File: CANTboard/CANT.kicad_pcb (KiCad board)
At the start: 2 copper layers, 67.6 x 50.8 mm, 63 parts, among them J1 Conn_02x08_Odd_Even, J2 Screw_Terminal_01x02, J3 Screw_Terminal_01x04, J4 USB_C_Receptacle_USB2.0, P2 SWD, SW1 SW_SPST, U1 USBLC6-2SC6, U2 SN74LVC1G14DBV, U3 ST485EBDR, U4 LD1117S33TR, U5 STM32H743VITx, U6 MCP2558FD-xSN, U7 74LVC1G66, U8 MCP2558FD-xSN, U9 74LVC1G66, Y1 Crystal

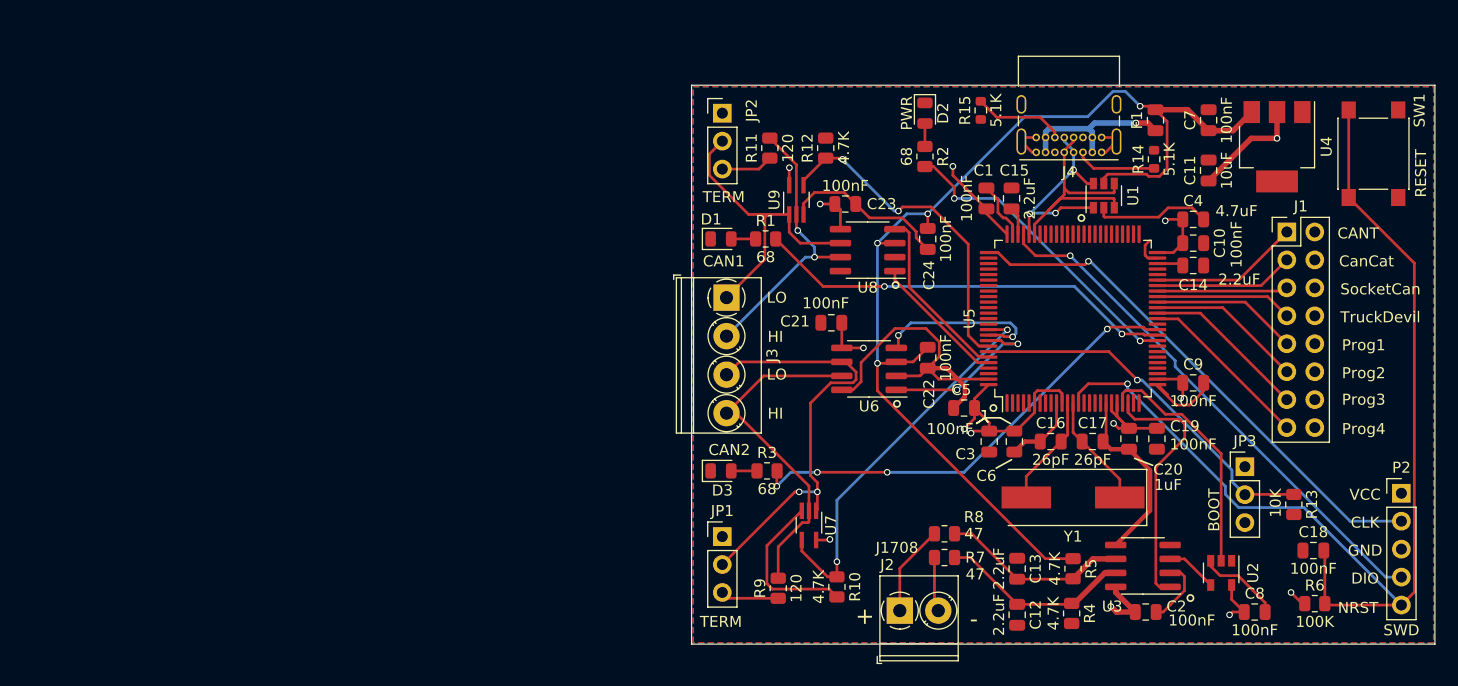
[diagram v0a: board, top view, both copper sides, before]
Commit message: Everything routed, commiting before last check before ordering PCBs
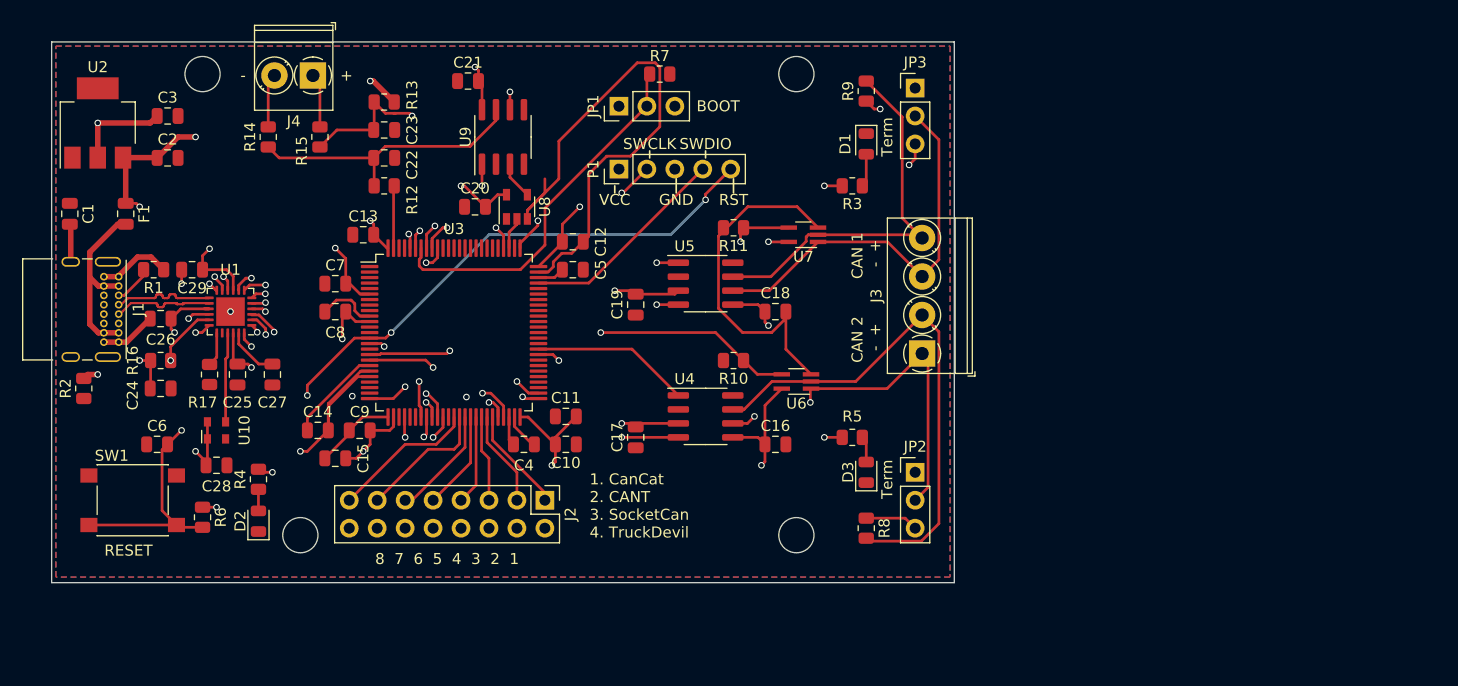
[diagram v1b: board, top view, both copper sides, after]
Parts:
- removed P2: SWD, Connector_PinHeader_2.54mm:PinHeader_1x05_P2.54mm_Vertical
- removed Y1: Crystal, Crystal:Crystal_SMD_HC49-SD
- added  : MountingHole_3.2mm_M3, MountingHole:MountingHole_3.2mm_M3, F.Cu at (37.5, 107.3)
- added  : MountingHole_3.2mm_M3, MountingHole:MountingHole_3.2mm_M3, F.Cu at (82.5, 107.3)
- added  : MountingHole_3.2mm_M3, MountingHole:MountingHole_3.2mm_M3, F.Cu at (82.5, 65.4)
- added  : MountingHole_3.2mm_M3, MountingHole:MountingHole_3.2mm_M3, F.Cu at (28.6, 65.4)
- added C25: 100nF, Capacitor_SMD:C_0805_2012Metric, F.Cu at (31.8, 92.7)
- added C26: 1uF, Capacitor_SMD:C_0805_2012Metric, F.Cu at (24.8, 87.6)
- added C27: 1uF, Capacitor_SMD:C_0805_2012Metric, F.Cu at (34.9, 92.7)
- added C28: 100nF, Capacitor_SMD:C_0805_2012Metric, F.Cu at (29.8, 101.0)
- added C29: 100nF, Capacitor_SMD:C_0805_2012Metric, F.Cu at (27.6, 83.2)
- added P1: SWD, Connector_PinHeader_2.54mm:PinHeader_1x05_P2.54mm_Vertical, F.Cu at (66.4, 74.0)
- added R16: 20K, Resistor_SMD:R_0805_2012Metric, F.Cu at (24.8, 91.4)
- added R17: 8.06K, Resistor_SMD:R_0805_2012Metric, F.Cu at (29.2, 92.7)
- added U10: DSC1001, DSC1001:Oscillator_SMD_Microchip_DSC1001-4Pin_2.5x2.0mm, F.Cu at (29.8, 97.8)
- C1: value 100nF -> 1uF
- C11: value 10uF -> 4.7uF
- C12, C13, C14: value 2.2uF -> 100nF
- C15: value 2.2uF -> 1uF
- C16, C17: value 26pF -> 100nF
- C20: value 1uF -> 100nF
- C22, C23, C5: value 100nF -> 2.2uF
- C24: value 100nF -> 4.7uF
- C3: value 100nF -> 10uF
- C4: value 4.7uF -> 2.2uF
- J1: value Conn_02x08_Odd_Even -> USB_C_Receptacle_USB2.0; footprint Connector_PinHeader_2.54mm:PinHeader_2x08_P2.54mm_Vertical -> Connector_USB:USB_C_Receptacle_GCT_USB4085
- J2: value Screw_Terminal_01x02 -> Conn_02x08_Odd_Even; footprint TerminalBlock_Phoenix:TerminalBlock_Phoenix_PT-1,5-2-3.5-H_1x02_P3.50mm_Horizontal -> Connector_PinHeader_2.54mm:PinHeader_2x08_P2.54mm_Vertical
- J4: value USB_C_Receptacle_USB2.0 -> Screw_Terminal_01x02; footprint Connector_USB:USB_C_Receptacle_GCT_USB4085 -> TerminalBlock_Phoenix:TerminalBlock_Phoenix_PT-1,5-2-3.5-H_1x02_P3.50mm_Horizontal
- R1, R2: value 68 -> 5.1K
- R11: value 120 -> 4.7K
- R13: value 10k -> 4.7K
- R14, R15: value 5.1K -> 47; footprint Resistor_SMD:R_0603_1608Metric -> Resistor_SMD:R_0805_2012Metric
- R4, R5: value 4.7K -> 68
- R7: value 47 -> 10k
- R8: value 47 -> 120
- U1: value USBLC6-2SC6 -> USB3343; footprint Package_TO_SOT_SMD:SOT-23-6 -> Package_DFN_QFN:QFN-24-1EP_4x4mm_P0.5mm_EP2.6x2.6mm
- U2: value SN74LVC1G14DBV -> LD1117S33TR; footprint Package_TO_SOT_SMD:SOT-23-5 -> Package_TO_SOT_SMD:SOT-223
- U3: value ST485EBDR -> STM32H743VITx; footprint Package_SO:SOIC-8_3.9x4.9mm_P1.27mm -> Package_QFP:LQFP-100_14x14mm_P0.5mm
- U4: value LD1117S33TR -> MCP2558FD-xSN; footprint Package_TO_SOT_SMD:SOT-223 -> Package_SO:SOIC-8_3.9x4.9mm_P1.27mm
- U5: value STM32H743VITx -> MCP2558FD-xSN; footprint Package_QFP:LQFP-100_14x14mm_P0.5mm -> Package_SO:SOIC-8_3.9x4.9mm_P1.27mm
- U6: value MCP2558FD-xSN -> 74LVC1G66; footprint Package_SO:SOIC-8_3.9x4.9mm_P1.27mm -> Package_TO_SOT_SMD:SOT-353_SC-70-5_Handsoldering
- U8: value MCP2558FD-xSN -> SN74LVC1G14DBV; footprint Package_SO:SOIC-8_3.9x4.9mm_P1.27mm -> Package_TO_SOT_SMD:SOT-23-5
- U9: value 74LVC1G66 -> ST485EBDR; footprint Package_TO_SOT_SMD:SOT-353_SC-70-5_Handsoldering -> Package_SO:SOIC-8_3.9x4.9mm_P1.27mm
- moved SW1 117.1 mm to (22.2, 104.1), turned to 0 degrees
- moved U2 110.0 mm to (19.1, 69.8), turned to 90 degrees
- moved J1 106.2 mm to (21.0, 83.8), turned to 270 degrees
- moved R6 101.4 mm to (28.6, 105.7), turned to 270 degrees
- moved C2 98.0 mm to (25.4, 73.0), turned to 0 degrees
- moved F1 94.0 mm to (21.6, 78.1), turned to 270 degrees
- moved R13 90.4 mm to (45.1, 67.9), turned to 180 degrees
- moved C8 87.9 mm to (40.6, 87.0)
- moved C1 83.3 mm to (16.5, 78.1), turned to 270 degrees
- moved G*** 82.4 mm to (33.0, 85.7)
- moved C14 81.0 mm to (39.1, 97.8)
- moved C7 80.8 mm to (40.6, 84.5), turned to 0 degrees
- moved R14 80.5 mm to (34.5, 71.1)
- moved C3 80.3 mm to (25.4, 69.2), turned to 0 degrees
- moved U1 80.1 mm to (31.1, 87.0), turned to 180 degrees
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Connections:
- C1 pad 1: VCC -> GND
- C1 pad 2: GND -> Net-(C1-Pad2)
- C10 pad 1: VCC -> GND
- C10 pad 2: GND -> VCC
- C11 pad 1: VCC -> GND
- C11 pad 2: GND -> VCC
- C12 pad 1: Net-(C12-Pad1) -> GND
- C12 pad 2: GND -> VCC
- C13 pad 2: Net-(C13-Pad2) -> VCC
- C14 pad 1: Net-(C14-Pad1) -> GND
- C14 pad 2: GND -> VCC
- C15 pad 1: Net-(C15-Pad1) -> GND
- C15 pad 2: GND -> VCC
- C16 pad 1: GND -> VCC
- C16 pad 2: Net-(C16-Pad2) -> GND
- C17 pad 1: Net-(C17-Pad1) -> GND
- C17 pad 2: GND -> VBUS
- C18 pad 1: GND -> VCC
- C18 pad 2: /NRST -> GND
- C19 pad 2: VCC -> VBUS
- C2 pad 1: GND -> VBUS
- C2 pad 2: VCC -> GND
- C22 pad 1: GND -> Net-(C22-Pad1)
- C22 pad 2: VBUS -> GND
- C23 pad 2: VCC -> Net-(C23-Pad2)
- C4 pad 1: VCC -> Net-(C4-Pad1)
- C5 pad 1: VCC -> Net-(C5-Pad1)
- C6 pad 1: VCC -> GND
- C6 pad 2: GND -> /Microcontroller/NRST
- C7 pad 1: VBUS -> GND
- C7 pad 2: GND -> VCC
- C8 pad 1: VCC -> GND
- C8 pad 2: GND -> VCC
- C9 pad 1: VCC -> GND
- C9 pad 2: GND -> VCC
- F1 pad 1: Net-(F1-Pad1) -> VBUS
- F1 pad 2: VBUS -> Net-(F1-Pad2)
- J2 pad 2: Net-(J2-Pad2) -> VCC
- J3 pad 1: CAN1_L -> CAN3_L
- J3 pad 2: CAN1_H -> CAN3_H
- J3 pad 3: CAN2_L -> CAN1_L
- J3 pad 4: CAN2_H -> CAN1_H
- JP1 pad 1: Net-(JP1-Pad1) -> (no net)
- JP1 pad 2: CAN2_L -> BOOT0
- JP1 pad 3: Net-(JP1-Pad3) -> VCC
- JP2 pad 1: Net-(JP2-Pad1) -> (no net)
- JP2 pad 2: CAN1_L -> CAN3_L
- JP3 pad 1: Net-(JP3-Pad1) -> (no net)
- JP3 pad 2: BOOT0 -> CAN1_L
- JP3 pad 3: VCC -> Net-(JP3-Pad3)
- R1 pad 1: Net-(D1-Pad2) -> GND
- R1 pad 2: LED_ACT1 -> Net-(J1-PadA5)
- R10 pad 1: CAN2_SHORT -> CAN3_SHORT
- R11 pad 1: Net-(JP2-Pad3) -> CAN1_SHORT
- R11 pad 2: CAN1_H -> GND
- R12 pad 1: CAN1_SHORT -> Net-(C22-Pad1)
- R13 pad 1: BOOT0 -> VBUS
- R13 pad 2: GND -> Net-(C23-Pad2)
- R14 pad 1: Net-(J4-PadA5) -> Net-(C22-Pad1)
- R14 pad 2: GND -> Net-(J4-Pad2)
- R15 pad 1: GND -> Net-(C23-Pad2)
- R15 pad 2: Net-(J4-PadB5) -> Net-(J4-Pad1)
- R2 pad 1: Net-(D2-Pad2) -> GND
- R2 pad 2: LED_PWR1 -> Net-(J1-PadB5)
- R3 pad 1: Net-(D3-Pad2) -> Net-(D1-Pad2)
- R3 pad 2: LED_ACT2 -> LED_ACT1
- R4 pad 1: Net-(C12-Pad1) -> Net-(D2-Pad2)
- R4 pad 2: GND -> LED_PWR1
- R5 pad 1: VBUS -> Net-(D3-Pad2)
- R5 pad 2: Net-(C13-Pad2) -> LED_ACT2
- R6 pad 2: /NRST -> /Microcontroller/NRST
- R7 pad 1: Net-(C12-Pad1) -> BOOT0
- R7 pad 2: Net-(J2-Pad2) -> GND
- R8 pad 1: Net-(C13-Pad2) -> Net-(JP2-Pad3)
- R8 pad 2: Net-(J2-Pad1) -> CAN3_H
- R9 pad 1: Net-(JP1-Pad3) -> Net-(JP3-Pad3)
- R9 pad 2: CAN2_H -> CAN1_H
- SW1 pad 2: /NRST -> /Microcontroller/NRST
- U1 pad 1: /USB_DP -> USB_DIR
- U1 pad 2: GND -> USB_CK
- U1 pad 3: /USB_DM -> USB_NXT
- U1 pad 4: /USB_DM -> USB_D0
- U1 pad 5: VBUS -> USB_D1
- U1 pad 6: /USB_DP -> USB_D2
- U2 pad 1: Net-(U2-Pad1) -> GND
- U2 pad 2: J1708_TX -> VCC
- U2 pad 3: GND -> VBUS
- U2 pad 4: Net-(U2-Pad4) -> (no net)
- U3 pad 1: J1708_RX -> (no net)
- U3 pad 2: GND -> (no net)
- U3 pad 3: Net-(U2-Pad4) -> (no net)
- U3 pad 4: GND -> (no net)
- U3 pad 5: GND -> (no net)
- U3 pad 6: Net-(C13-Pad2) -> VCC
- U3 pad 7: Net-(C12-Pad1) -> (no net)
- U3 pad 8: VCC -> (no net)
- U4 pad 1: GND -> CAN3_TX
- U4 pad 2: VCC -> GND
- U4 pad 4: (no net) -> CAN3_RX
- U5 pad 1: Net-(U5-Pad1) -> CAN1_TX
- U5 pad 2: Net-(U5-Pad2) -> GND
- U5 pad 3: Net-(U5-Pad3) -> VBUS
- U5 pad 4: Net-(U5-Pad4) -> CAN1_RX
- U5 pad 5: Net-(U5-Pad5) -> VCC
- U5 pad 6: VCC -> CAN1_L
- U5 pad 7: Net-(U5-Pad7) -> CAN1_H
- U5 pad 8: Net-(U5-Pad8) -> GND
- U6 pad 1: CAN2_TX -> CAN3_L
- U6 pad 2: GND -> CAN3_H
- U6 pad 3: VBUS -> GND
- U6 pad 4: CAN2_RX -> CAN3_SHORT
- U7 pad 1: CAN2_L -> CAN1_L
- U7 pad 2: CAN2_H -> CAN1_H
- U7 pad 4: CAN2_SHORT -> CAN1_SHORT
- U8 pad 1: CAN1_TX -> (no net)
- U8 pad 2: GND -> J1708_TX
- U8 pad 3: VBUS -> GND
- U8 pad 4: CAN1_RX -> Net-(U8-Pad4)
- U9 pad 1: CAN1_L -> J1708_RX
- U9 pad 2: CAN1_H -> GND
- U9 pad 3: GND -> Net-(U8-Pad4)
- U9 pad 4: CAN1_SHORT -> GND
- U9 pad 5: VCC -> GND
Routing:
- net /NRST: track 99.4 -> 0.00 mm, vias 1 -> 0
- net /Microcontroller/NRST: track 0.00 -> 80.9 mm, vias 0 -> 4
- net /SWDIO: track 48.1 -> 0.00 mm, vias 1 -> 0
- net /SWCLK: track 47.9 -> 0.00 mm, vias 1 -> 0
- net CAN3_H: track 0.00 -> 47.7 mm
- net CAN2_L: track 39.8 -> 0.00 mm, vias 2 -> 0
- net USB_D7: track 0.00 -> 38.6 mm, vias 0 -> 2
- net CAN3_SHORT: track 0.00 -> 38.6 mm, vias 0 -> 2
- net USB_D6: track 0.00 -> 36.8 mm, vias 0 -> 2
- net USB_STP: track 0.00 -> 36.4 mm, vias 0 -> 2
- net USB_D5: track 0.00 -> 36.1 mm, vias 0 -> 2
- net CAN2_SHORT: track 35.7 -> 0.00 mm, vias 2 -> 0
- net USB_D2: track 0.00 -> 35.7 mm, vias 0 -> 2
- net USB_D3: track 0.00 -> 35.6 mm, vias 0 -> 2
- net USB_DIR: track 0.00 -> 35.5 mm, vias 0 -> 2
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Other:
- board size 67.6 x 50.8 mm -> 82 x 49.1 mm
- copper layers 2 -> 4
- board text added: "1. CanCat 2. CANT 3. SocketCan 4. TruckDevil"
- board text added: "8 7 6 5 4 3 2 1"
- board text added: "CAN 1 - +"
- board text added: "CAN 2 - +"
- board text added: "RST"
- board text added: "SWCLK"
- board text added: "SWDIO"
- board text added: "Term"
- board text removed: "100K"
- board text removed: "100nF"
- board text removed: "10K"
- board text removed: "10uF"
- board text removed: "120"
- board text removed: "1uF"
- board text removed: "2.2uF"
- board text removed: "26pF"
- board text removed: "4.7K"
- board text removed: "4.7uF"
- board text removed: "47"
- board text removed: "5.1K"
- board text removed: "68"
- board text removed: "CAN1"
- board text removed: "CAN2"
- board text removed: "CANT"
- board text removed: "CLK"
- board text removed: "CanCat"
- board text removed: "DIO"
- board text removed: "HI"
- board text removed: "J1708"
- board text removed: "LO"
- board text removed: "NRST"
- board text removed: "PWR"
- board text removed: "Prog1"
- board text removed: "Prog2"
- board text removed: "Prog3"
- board text removed: "Prog4"
- board text removed: "SWD"
- board text removed: "SocketCan"
- board text removed: "TERM"
- board text removed: "TruckDevil"
